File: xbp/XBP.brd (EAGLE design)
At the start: 61.3 x 31.1 mm, 41 parts, among them IC1 MCP1701AT, Q1 BSS84, Q2 BSS123, Q3 BSS123, Q4 BSS123, Q5 BSS123, Q6 BSS123, Q7 BSS123, Q8 BSS123, U1 INA225, U3 SILK_3V3_TAG, U4 SILK_3V3_TAG, X1 SMA-142-0711-871/876

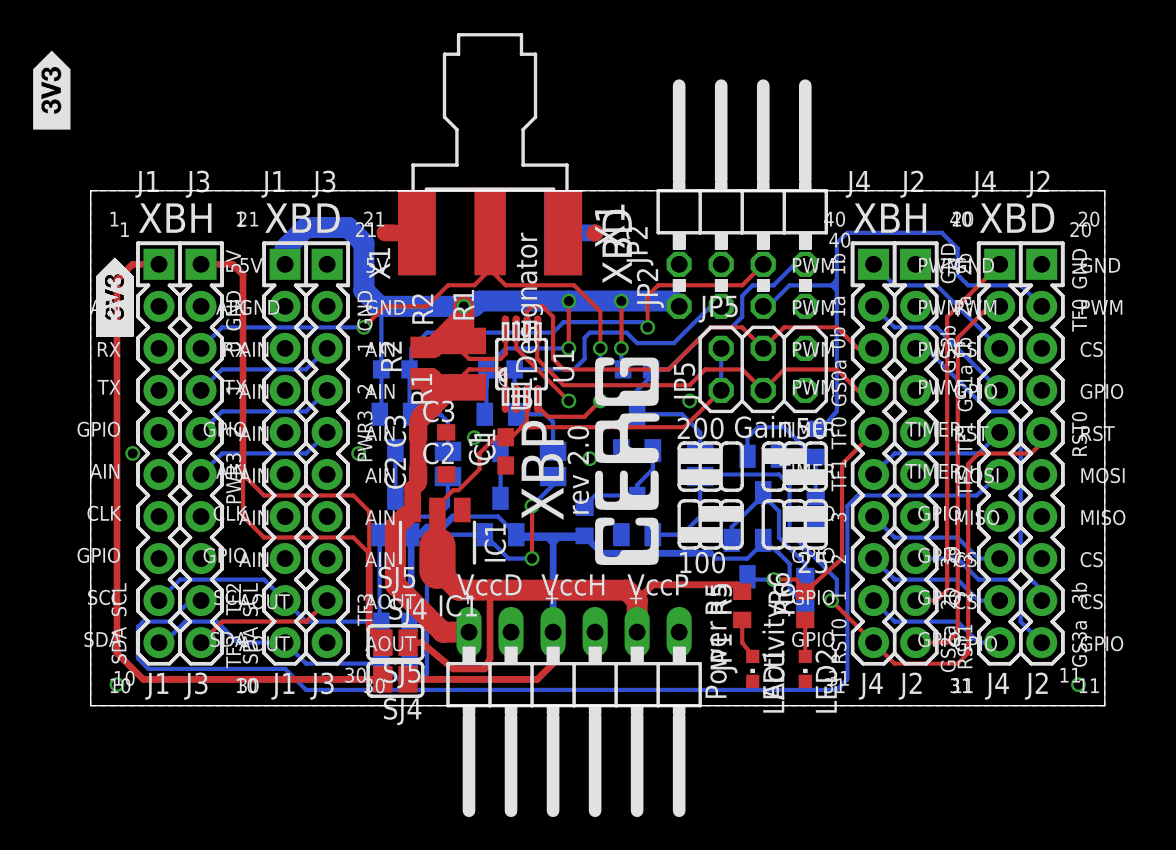
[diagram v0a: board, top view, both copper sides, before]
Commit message: XBP version 2.1
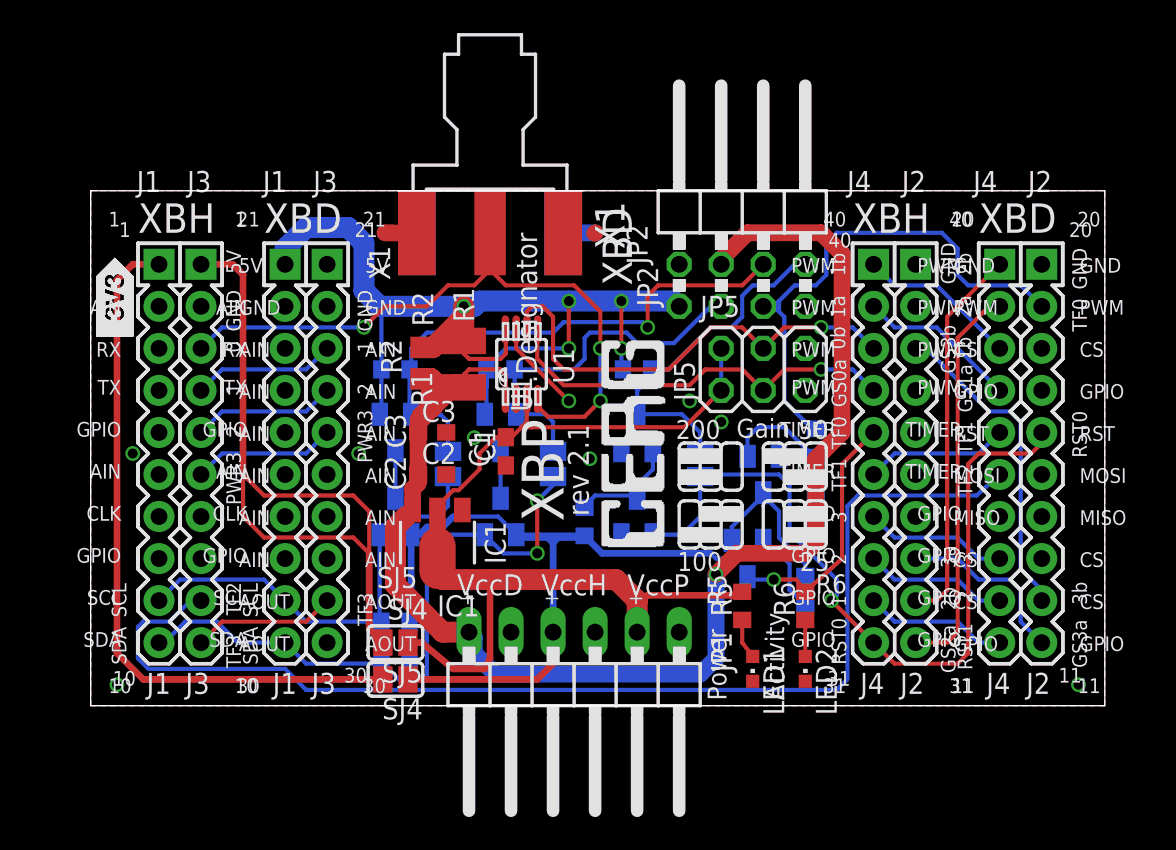
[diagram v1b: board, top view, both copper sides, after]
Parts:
- removed U4: SILK_3V3_TAG, Public_BP_Library:SILK_3V3_TAG
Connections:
- net VCCXBD: now also JP2.4
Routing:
- net VCCXBD: track 31.5 -> 87.2 mm, vias 0 -> 1
- net TF0D: track 32.8 -> 31.8 mm
- net GS1: vias 0 -> 1
- net GS0: vias 0 -> 1
- net GND: vias 8 -> 9
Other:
- board text added: "VIN"
- board text added: "XXBX Power Shim-XBP"
- board text added: "rev 2.1"
- board text removed: "rev 2.0"
